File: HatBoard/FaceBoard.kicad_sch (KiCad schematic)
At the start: 18 parts, among them J1 Molex FC Connection, J2 DF11 FC Connection, J3 Conn_01x04, U1 VEML7700, U2 DRV2605LDGS, U25 TMP112AIDRLR, U4 TCA4311A

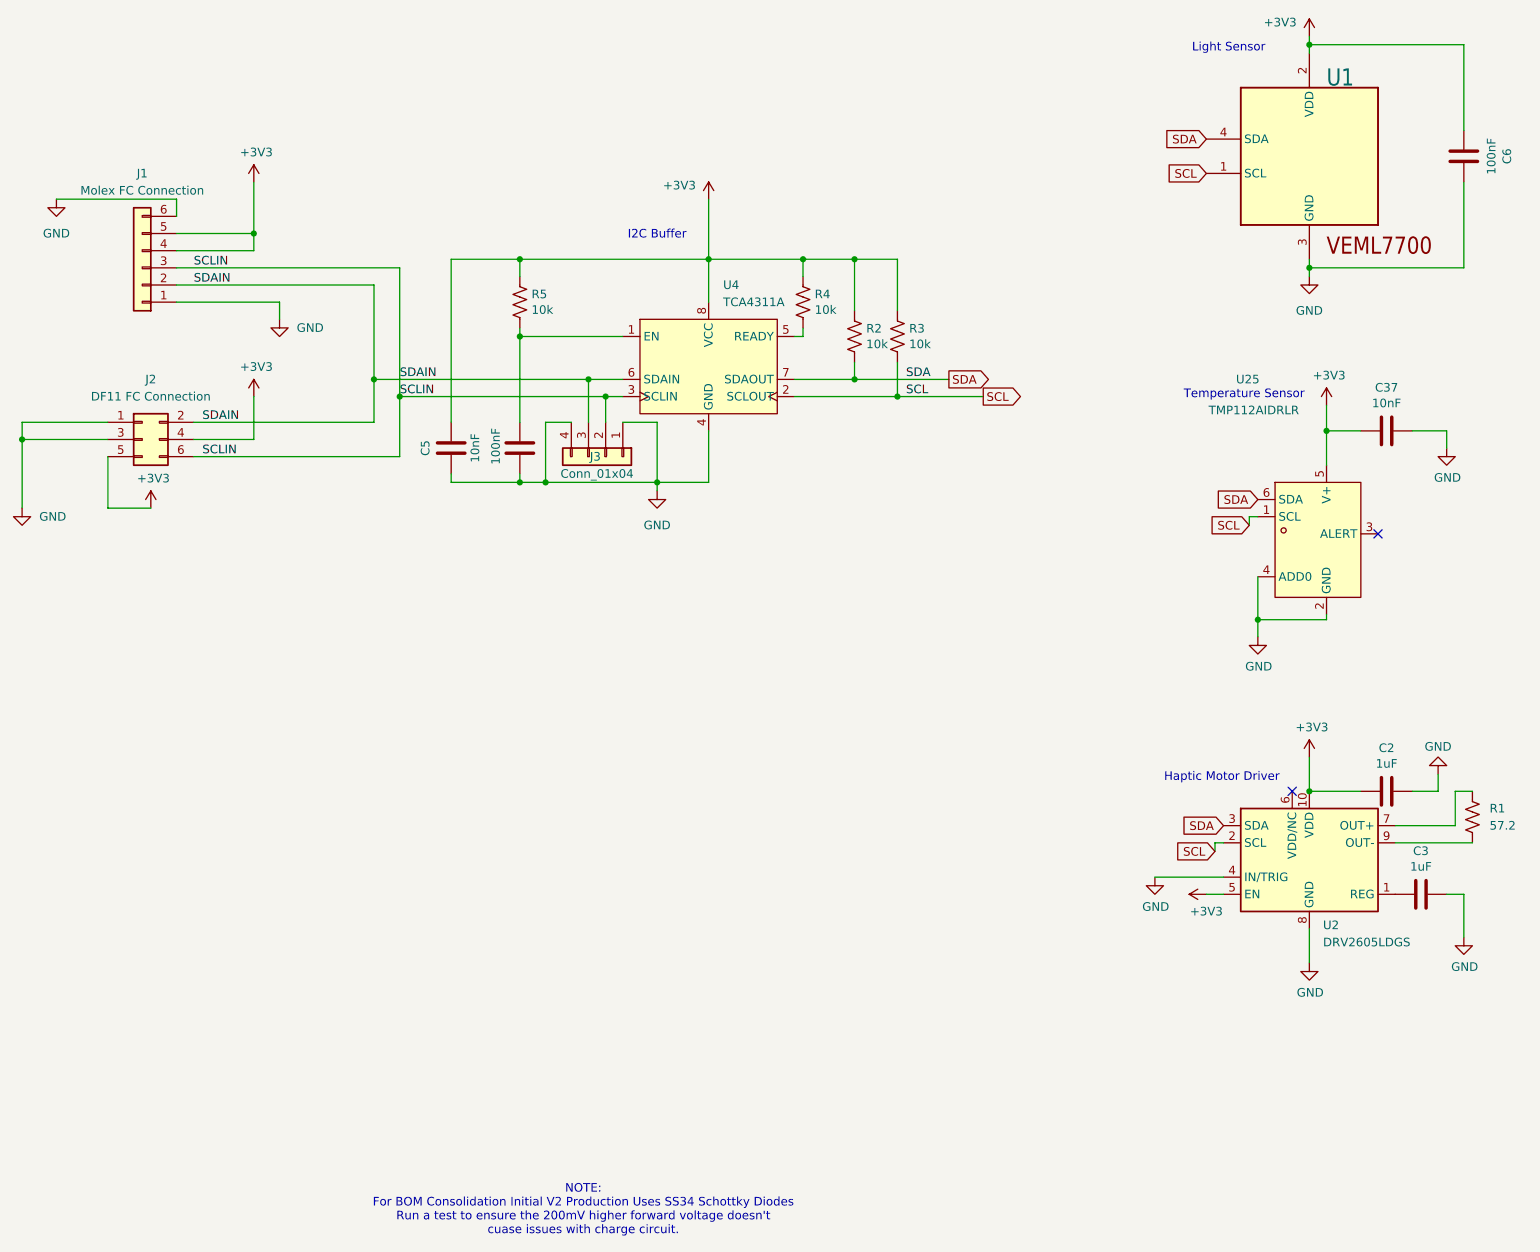
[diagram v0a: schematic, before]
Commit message: new everything should be here
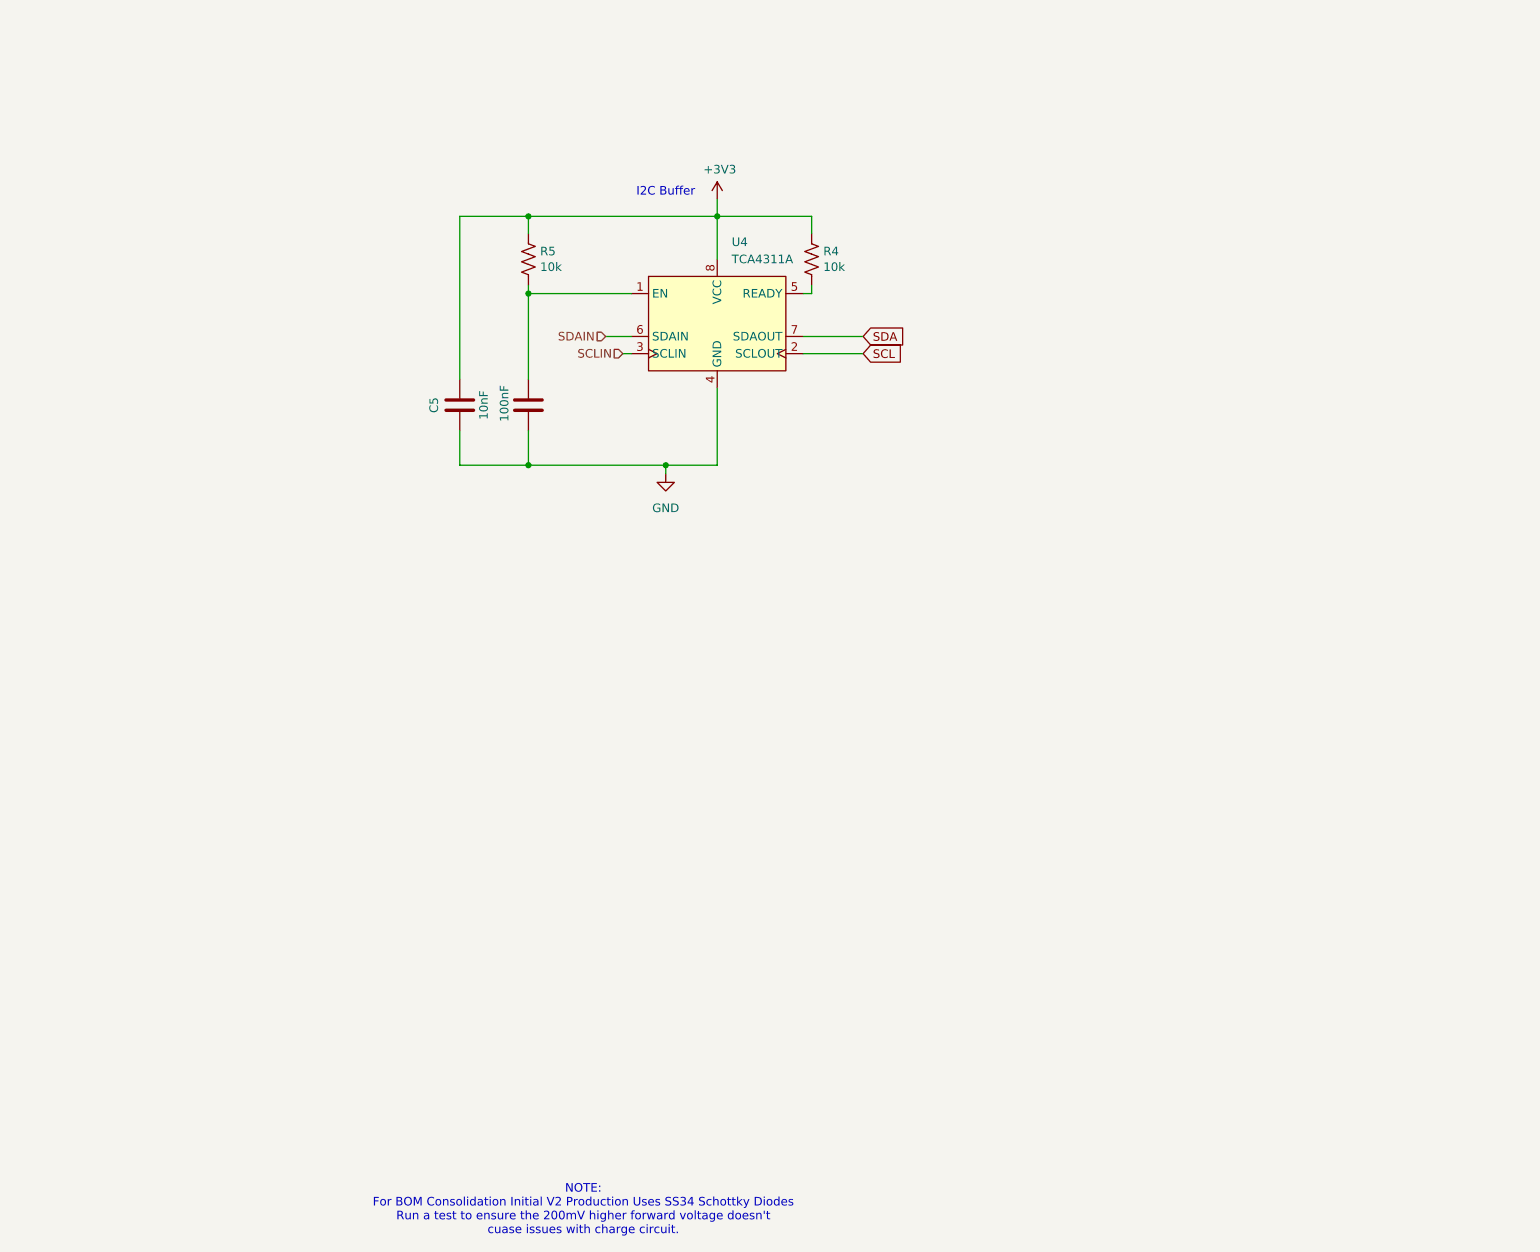
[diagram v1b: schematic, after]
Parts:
- removed C2, C3: 1uF, Capacitor_SMD:C_0805_2012Metric, symbol Device:C
- removed C37: 10nF, Capacitor_SMD:C_0402_1005Metric, symbol Device:C
- removed C6: 100nF, Capacitor_SMD:C_0402_1005Metric, symbol Device:C
- removed J1: Molex FC Connection, easyeda2kicad:CONN-SMD_6P-P1.50_A1501WRB-S-6P, symbol Connector_Generic:Conn_01x06
- removed J2: DF11 FC Connection, Connector_Hirose:Hirose_DF11-6DP-2DSA_2x03_P2.00mm_Vertical, symbol Connector_Generic:Conn_02x03_Odd_Even
- removed J3: Conn_01x04, Connector_PinHeader_2.00mm:PinHeader_1x04_P2.00mm_Vertical, symbol Connector_Generic:Conn_01x04
- removed R1: 57.2, Resistor_SMD:R_0201_0603Metric_Pad0.64x0.40mm_HandSolder, symbol Device:R_US
- removed R2, R3: 10k, Resistor_SMD:R_0603_1608Metric, symbol Device:R_US
- removed U1: VEML7700, easyeda2kicad:SENSOR-SMD_EML7700-TT, symbol Adafruit VEML7700-eagle-import:VEML7700
- removed U2: DRV2605LDGS, Package_SO:VSSOP-10_3x3mm_P0.5mm, symbol Driver_Haptic:DRV2605LDGS
- removed U25: TMP112AIDRLR, easyeda2kicad:SOT-563_L1.6-W1.2-P0.50-LS1.6-BR, symbol easyeda2kicad:TMP112AIDRLR
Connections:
- net SCLIN: no longer U4.6 (SDAIN)
- new net SDAIN: U4.6 (SDAIN)
- no-connect marks 2 -> 0
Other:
- note removed: "Haptic Motor Driver"
- note removed: "Light Sensor"
- note removed: "Temperature Sensor"
- moved on the sheet: C5, R4, R5, U4
